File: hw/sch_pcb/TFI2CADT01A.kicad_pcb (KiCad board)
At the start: 2 copper layers, 25 x 15 mm, 25 parts, among them J1 SM04B-GHS-TB, J2 SM04B-GHS-TB, J3 SM04B-GHS-TB, J4 SM04B-GHS-TB, M1 HOLE, M2 HOLE, M3 HOLE, M4 HOLE, M5 HOLE, M6 HOLE, U1 MIC5504-3.3YM5, U2 TCA4307

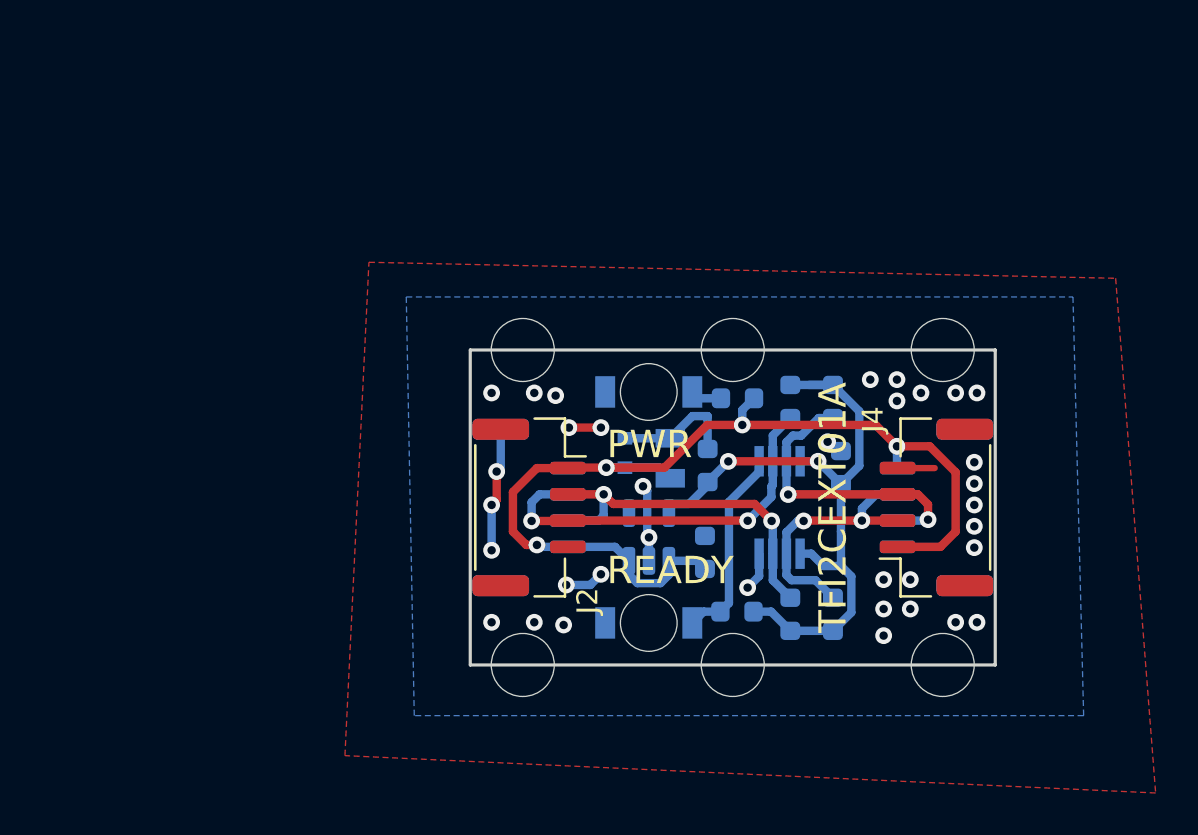
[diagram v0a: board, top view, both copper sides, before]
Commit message: Edit PCB
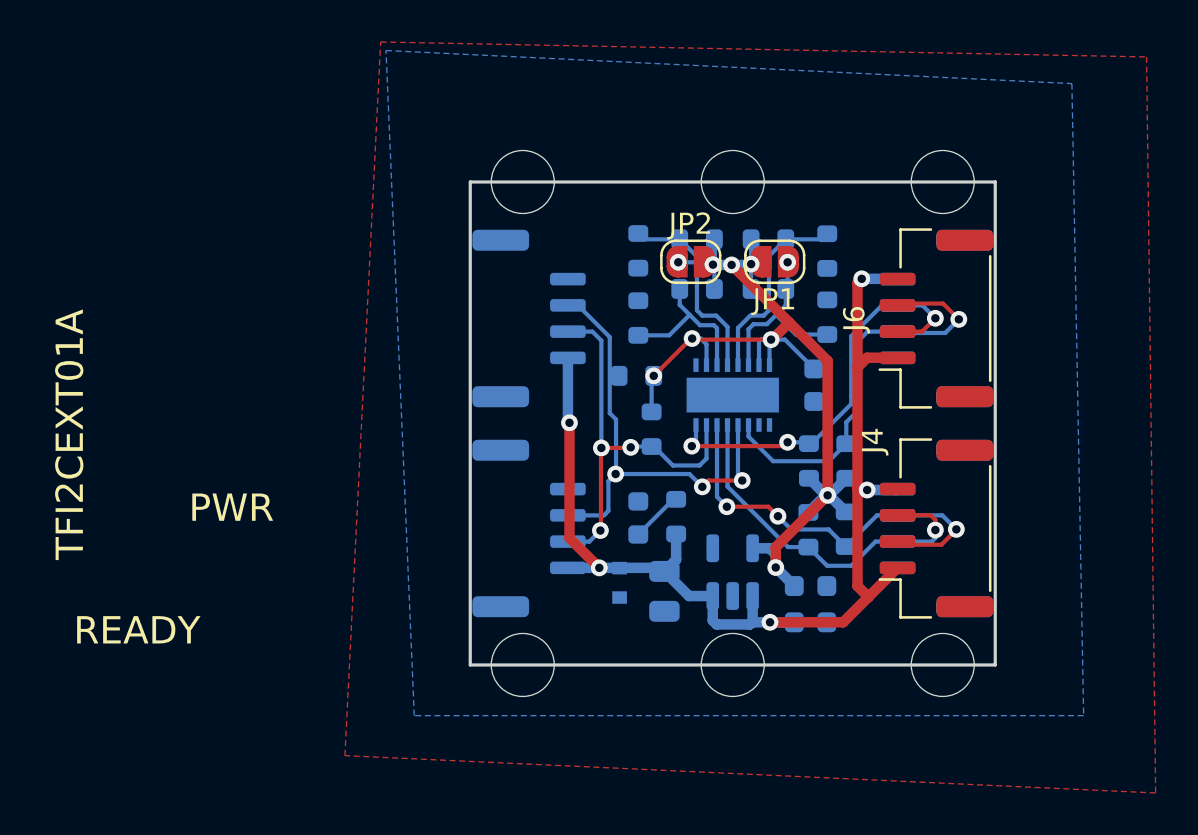
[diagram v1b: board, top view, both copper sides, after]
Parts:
- removed D3: LED RED, Mlab_D:LED_1206
- removed R4: 180R, Mlab_R:SMD-0603
- added J5: SM04B-GHS-TB, Connector_JST:JST_GH_SM04B-GHS-TB_1x04-1MP_P1.25mm_Horizontal, B.Cu at (22.2, -16.5)
- added J6: SM04B-GHS-TB, Connector_JST:JST_GH_SM04B-GHS-TB_1x04-1MP_P1.25mm_Horizontal, F.Cu at (22.2, -16.5)
- added JP1: SolderJumper_2_Open, Jumper:SolderJumper-2_P1.3mm_Open_RoundedPad1.0x1.5mm, F.Cu at (14.5, -19.2)
- added JP2: SolderJumper_2_Open, Jumper:SolderJumper-2_P1.3mm_Open_RoundedPad1.0x1.5mm, F.Cu at (10.5, -19.2)
- added R10: 1M, Resistor_SMD:R_0603_1608Metric, B.Cu at (17.0, -16.6)
- added R12: 1M, Resistor_SMD:R_0603_1608Metric, B.Cu at (10.8, -17.9)
- added R13: 887k, Resistor_SMD:R_0603_1608Metric, B.Cu at (8.00, -16.5)
- added R14: 887k, Resistor_SMD:R_0603_1608Metric, B.Cu at (10.8, -20.3)
- added R15: 1M, Resistor_SMD:R_0603_1608Metric, B.Cu at (8.00, -19.7)
- added R16: 10k, Resistor_SMD:R_0603_1608Metric, B.Cu at (16.1, -9.71)
- added R17: 10k, Resistor_SMD:R_0603_1608Metric, B.Cu at (17.9, -9.71)
- added R7: -, Resistor_SMD:R_0603_1608Metric, B.Cu at (14.2, -20.3)
- added R8: 180R, Resistor_SMD:R_0603_1608Metric, B.Cu at (17.0, -19.7)
- added R9: 887k, Resistor_SMD:R_0603_1608Metric, B.Cu at (14.2, -17.9)
- C1: footprint Mlab_R:SMD-0805 -> Capacitor_SMD:C_0805_2012Metric
- C2, C3, C4: footprint Mlab_R:SMD-0603 -> Capacitor_SMD:C_0603_1608Metric
- D1: footprint Mlab_D:LED_1206 -> LED_SMD:LED_0603_1608Metric
- J2: moved to B.Cu
- R1, R2, R3, R5, R6: footprint Mlab_R:SMD-0603 -> Resistor_SMD:R_0603_1608Metric
- U2: value TCA4307 -> LTC4317; footprint Package_SO:VSSOP-8_3.0x3.0mm_P0.65mm -> Package_DFN_QFN:DFN-16-1EP_3x5mm_P0.5mm_EP1.66x4.4mm
- moved R2 11.0 mm to (8.64, -11.2), turned to -90 degrees
- moved J2 9.00 mm to (2.80, -16.5), turned to 90 degrees
- moved M2 8.00 mm to (12.5, -23.0)
- moved M4 8.00 mm to (2.50, -23.0)
- moved M5 8.00 mm to (22.5, -23.0)
- moved C3 7.55 mm to (16.2, -3.76), turned to 0 degrees
- moved R3 7.43 mm to (7.91, -13.8), turned to 180 degrees
- moved R1 6.35 mm to (9.80, -7.06), turned to 90 degrees
- moved C1 6.34 mm to (9.25, -3.51), turned to -90 degrees
- moved R6 6.22 mm to (16.1, -6.44)
- moved D2 6.19 mm to (7.11, -3.91), turned to -90 degrees
- moved C2 6.03 mm to (16.2, -2.03), turned to 0 degrees
- moved D1 6.02 mm to (8.00, -7.00), turned to -90 degrees
- moved U2 5.80 mm to (12.5, -12.9), turned to -90 degrees
- moved U1 4.33 mm to (12.5, -4.42)
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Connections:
- J3 pad 2: /SCLout -> /SCLout1
- J3 pad 3: /SDAout -> /SDAout1
- J4 pad 2: /SCLout -> /SCLout1
- J4 pad 3: /SDAout -> /SDAout1
- R5 pad 2: /SCLout -> /SCLout1
- R6 pad 2: /SDAout -> /SDAout1
- U2 pad 1: +3V3 -> GND
- U2 pad 2: /SCLout -> +3V3
- U2 pad 3: /SCLin -> /XORH2
- U2 pad 4: GND -> /XORL2
- U2 pad 5: Net-(D3-Pad2) -> /XORH1
- U2 pad 6: /SDAin -> /XORL1
- U2 pad 7: /SDAout -> +3V3
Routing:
- net GND: track 23.4 -> 0.00 mm, vias 35 -> 0
- net /SCLout1: track 0.00 -> 20.5 mm, vias 0 -> 3
- net /SCLout2: track 0.00 -> 19.9 mm, vias 0 -> 3
- net /SDAout2: track 0.00 -> 19.7 mm, vias 0 -> 1
- net /SDAout1: track 0.00 -> 17.7 mm, vias 0 -> 1
- net +3V3: track 33.5 -> 49.8 mm, vias 2 -> 8
- net /SDAout: track 14.3 -> 0.00 mm, vias 2 -> 0
- net /SCLout: track 12.8 -> 0.00 mm, vias 2 -> 0
- net /XORL2: track 0.00 -> 10.4 mm, vias 0 -> 1
- net Net-(D3-Pad2): track 9.49 -> 0.00 mm
- net /XORH1: track 0.00 -> 9.39 mm
- net /XORL1: track 0.00 -> 8.91 mm, vias 0 -> 1
- net /XORH2: track 0.00 -> 7.61 mm
- net +5V: track 48.5 -> 55.0 mm, vias 4 -> 5
- net /SDAin: track 18.8 -> 22.8 mm, vias 2 -> 3
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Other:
- board size 25 x 15 mm -> 25 x 23 mm
